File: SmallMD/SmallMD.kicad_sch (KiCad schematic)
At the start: 180 parts, among them J1 Conn_01x02_Male, J2 Conn_01x02_Female, J3 Conn_01x10_Male, J4 Conn_01x02_Female, J5 Conn_01x04_Male, J6 Conn_01x04_Male, J7 Conn_01x10_Male, J8 Conn_01x06_Male, Q1 SSM6J808R, Q10 S8050, Q11 S8050, Q14 BSS138, Q15 BSS138, Q16 S8050, Q18 μPA2753GR, Q19 μPA2753GR, Q2 BSS138, Q3 SSM6J808R, Q4 SSM3J332R, Q5 SSM3J332R, Q6 S8050, Q7 S8050, Q8 SSM3J332R, Q9 SSM3J332R, SW1 SW_DIP_x05, SW2 SW_SPDT, SW3 SW_SPDT_White, SW4 SW_SPST, U1 AZ1084CD-3.3, U10 IR2302, U11 IR2302, U12 MAX3485, U2 AZ1084CD-5.0, U3 STM32C031K4T6, U4 MAX3485, U5 MAX3485, U6 LT6106, U7 MAX3485, U8 TLP2361, U9 TLP2361, Y1 48MHz

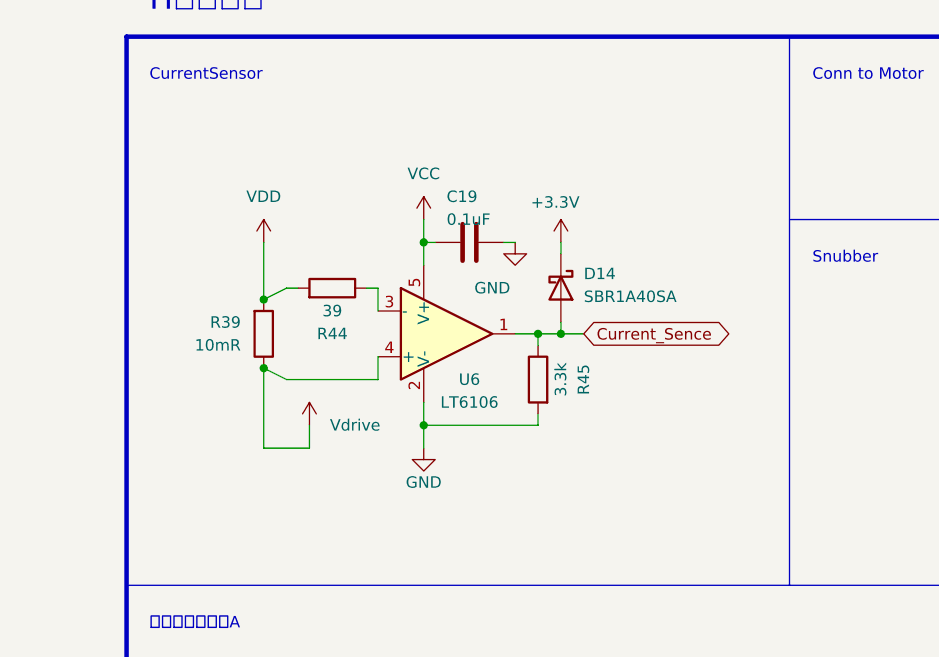
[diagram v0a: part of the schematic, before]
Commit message: 回路図pdf出力
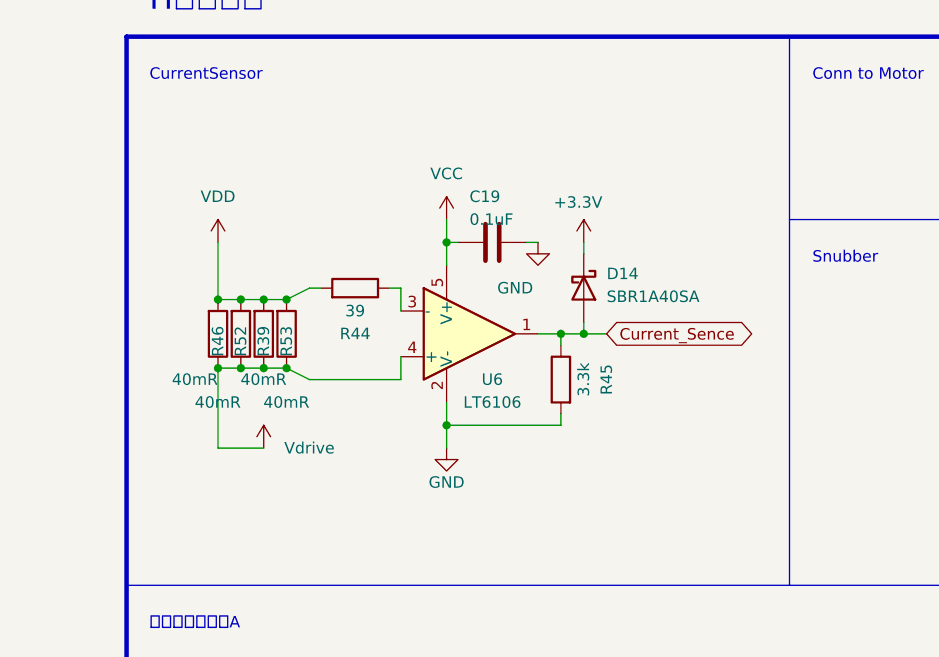
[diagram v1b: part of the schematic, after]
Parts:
- added R46, R52, R53: 40mR, Resistor_SMD:R_2512_6332Metric, symbol Device:R
- R39: value 10mR -> 40mR; footprint (none) -> Resistor_SMD:R_2512_6332Metric
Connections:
- net VDD: now also R46.2, R52.2, R53.2
- net Vdrive: now also R46.1, R52.1, R53.1
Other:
- moved on the sheet: C19, D14, R44, R45, U6
